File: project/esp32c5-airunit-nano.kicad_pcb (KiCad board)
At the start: 2 copper layers, 19.1 x 21.8 mm, 26 parts, among them J1 FPC0.5B-WTX-24P, J2 Conn_01x01_Pin, J4 Conn_01x01_Pin, J5 Conn_01x01_Pin, J6 Conn_01x01_Pin, J7 Conn_01x01_Pin, J8 TF-021B-H265, J9 Conn_01x01_Pin, SW1 EVQP7C01P, U1 MT3406, U2 ESP32-C5-WROOM-1U-N8R8, Y1 YD24MUBCE2O

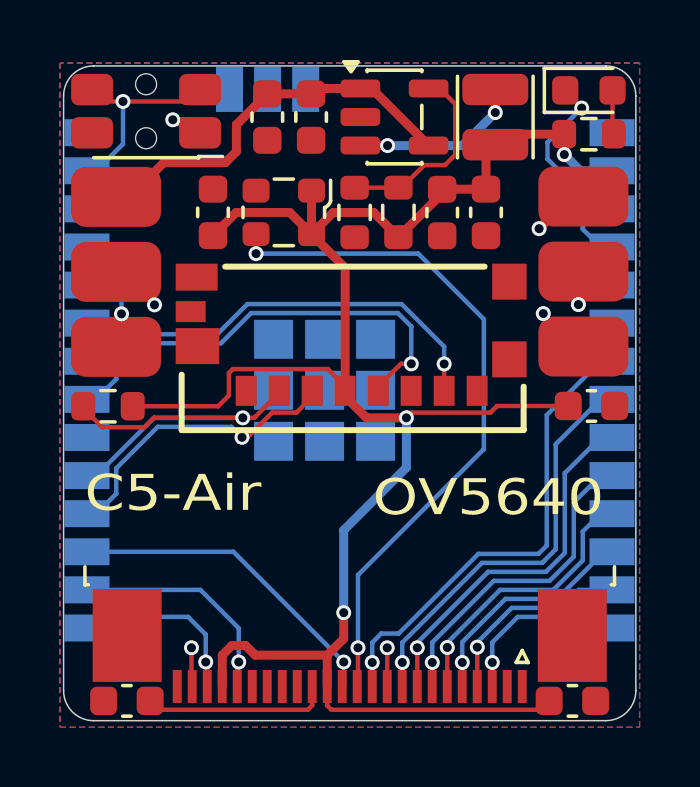
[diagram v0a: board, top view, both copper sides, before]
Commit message: i've updated the files
there were some major errors in the v1.0 of the project
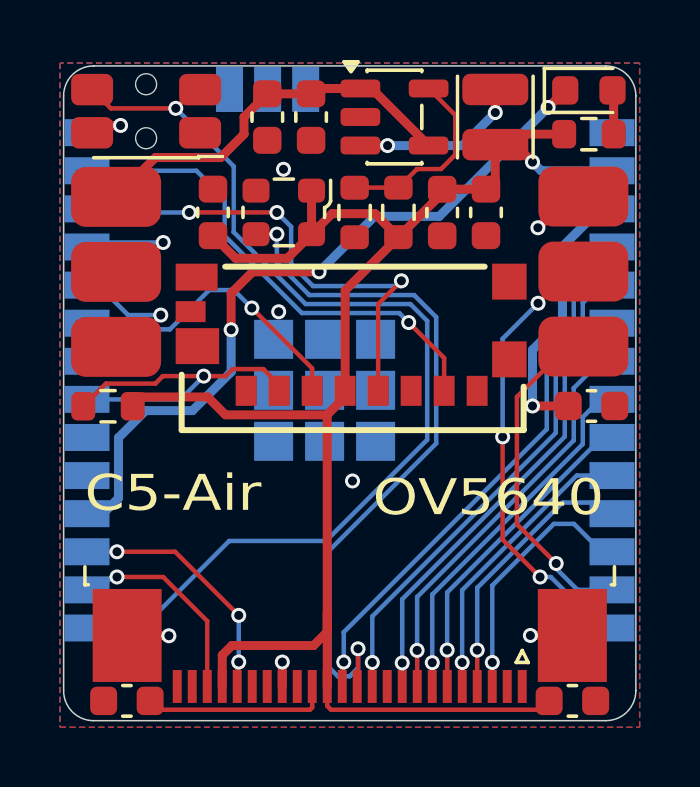
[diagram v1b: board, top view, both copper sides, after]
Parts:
- R1, R6: value 100kR -> 47kR
- R2: value 25kR -> 12kR
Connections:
- J1 pad 17: unconnected-(J1-Pin_17-Pad17) -> GND
- U2 pad 10: d4 -> d3
- U2 pad 11: d0 -> d1
- U2 pad 12: d3 -> d2
- U2 pad 13: d1 -> uart1_rx
- U2 pad 14: d2 -> uart1_tx
- U2 pad 15: sda -> record
- U2 pad 16: scl -> sda
- U2 pad 17: d7 -> scl
- U2 pad 18: sd_cmd -> led
- U2 pad 19: sd_cd -> unconnected-(U2-GPIO15-Pad19)
- U2 pad 21: sd_clk -> sd_cd
- U2 pad 23: sd_data -> sd_cmd
- U2 pad 26: unconnected-(U2-GPIO25-Pad26) -> sd_clk
- U2 pad 27: record -> sd_data
- U2 pad 3: unconnected-(U2-EN/CHIP_PU-Pad3) -> +3V0
- U2 pad 4: led -> d7
- U2 pad 5: uart1_tx -> d6
- U2 pad 6: uart1_rx -> d5
- U2 pad 7: d6 -> pclk
- U2 pad 8: d5 -> d4
- U2 pad 9: pclk -> d0
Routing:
- net record: track 6.92 -> 34.6 mm
- net led: track 7.03 -> 24.5 mm, vias 1 -> 3
- net uart1_tx: track 3.19 -> 15.2 mm, vias 1 -> 3
- net d7: track 10.9 -> 18.6 mm
- net uart1_rx: track 4.62 -> 11.3 mm
- net +3V0: track 64.3 -> 67.8 mm, vias 3 -> 2
- net d2: track 5.97 -> 8.59 mm
- net d1: track 6.69 -> 9.11 mm
- net d3: track 7.72 -> 9.79 mm
- net uart0_rx: track 2.99 -> 4.80 mm
- net sd_data: track 14.5 -> 16.3 mm
- net sd_cd: track 13.4 -> 11.7 mm
- net d0: track 9.30 -> 10.8 mm
- net d4: track 10.8 -> 12.3 mm
- net pclk: track 12.3 -> 13.8 mm
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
